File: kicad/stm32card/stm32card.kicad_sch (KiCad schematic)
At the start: 53 parts, among them J1 USB_C_Receptacle_PowerOnly_6P, Q1 AO3400A, U1 MT9216, U2 LM66100DCK, U3 LM66100DCK, U4 STM32F103C8T6, U5 N096-1608TBBIG11-H13

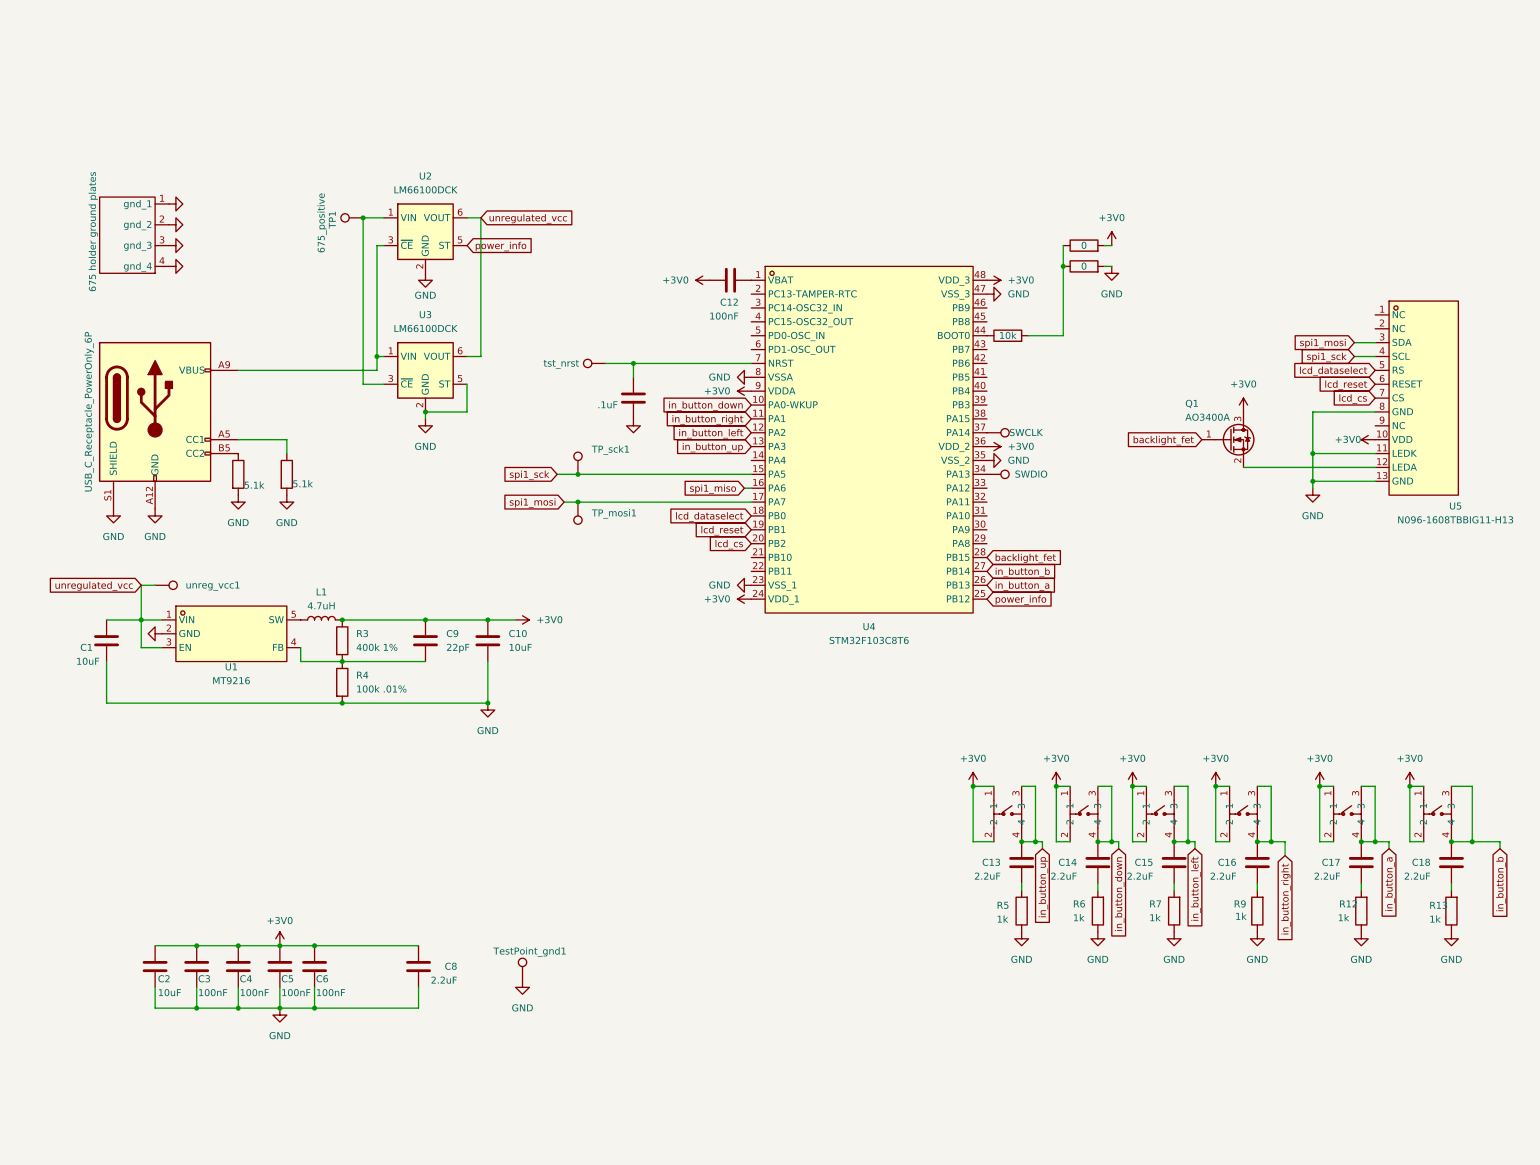
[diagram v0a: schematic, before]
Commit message: need to organize, redid PCB
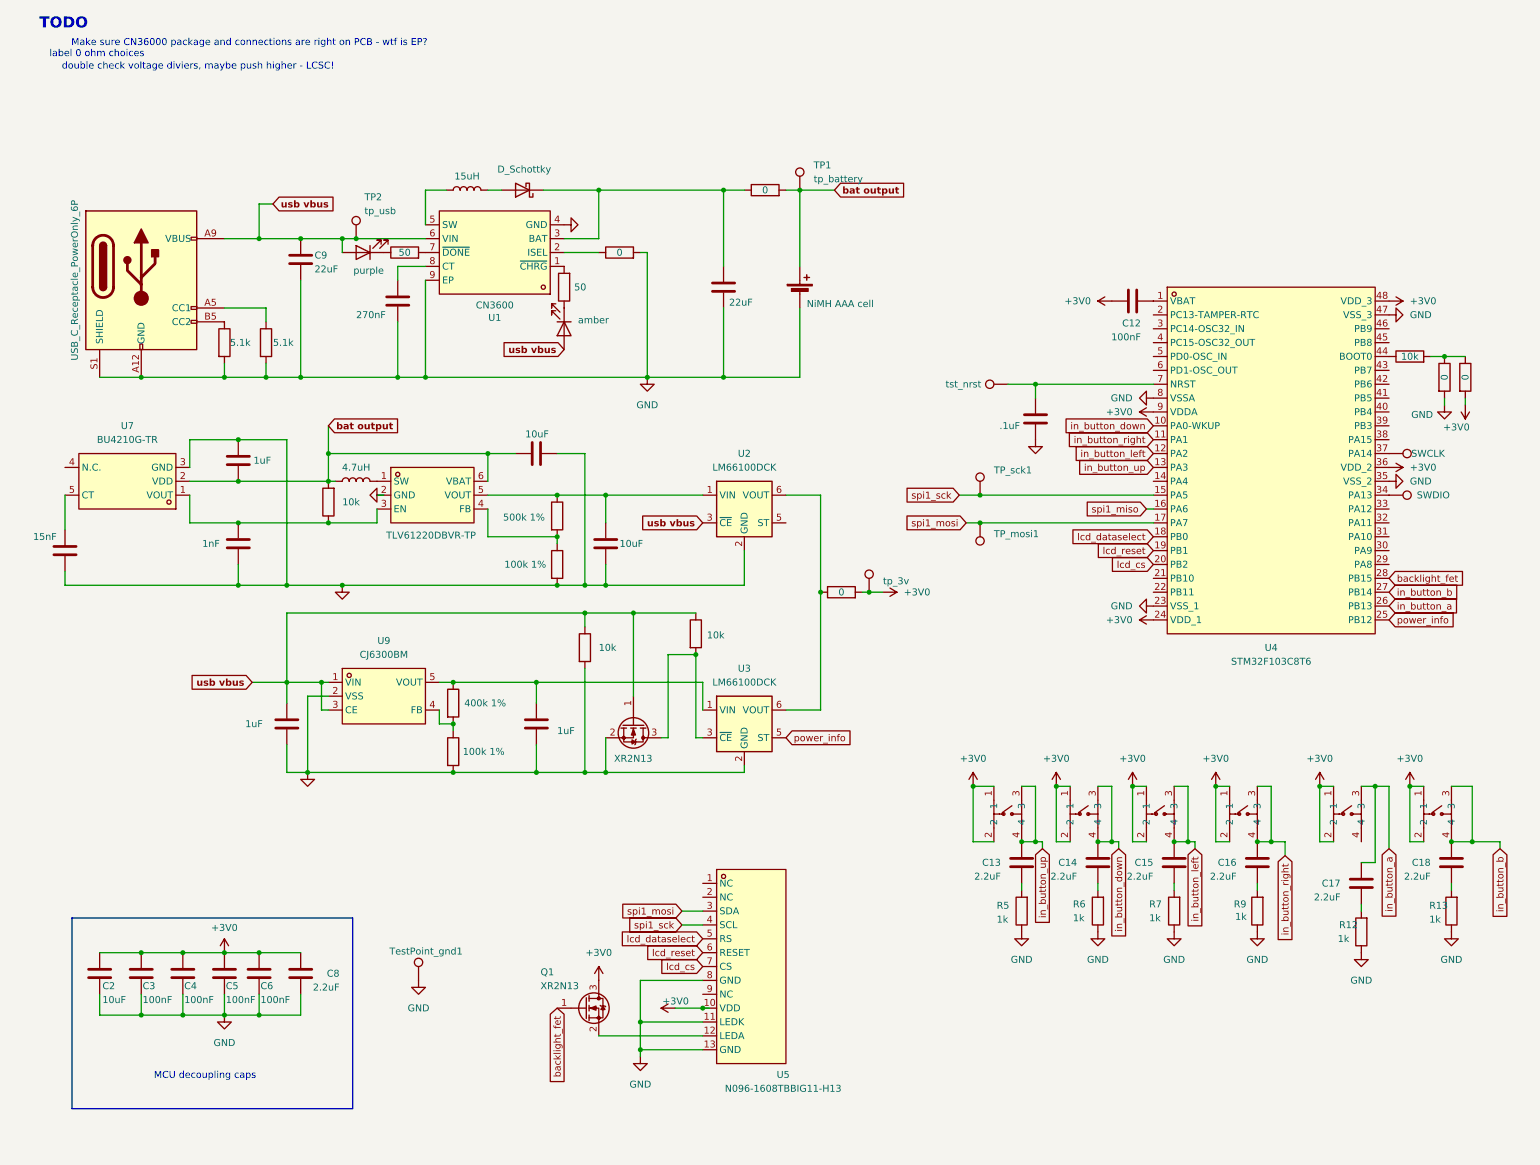
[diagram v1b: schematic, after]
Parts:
- removed R3: 400k 1%, Resistor_SMD:R_0805_2012Metric, symbol Device:R
- removed U1: MT9216, easyeda2kicad:SOT-23-5_L3.0-W1.7-P0.95-LS2.8-BL, symbol easyeda2kicad:MT9216
- removed U6: ~, Library:battery_holder, symbol battery_holder:quad_675
- removed unreg_vcc1: unreg_vcc, TestPoint:TestPoint_Pad_D2.0mm, symbol Connector:TestPoint
- added BT1: NiMH AAA cell, Battery:BatteryHolder_Keystone_2466_1xAAA, symbol Device:Battery_Cell
- added C19: 1nF, Capacitor_SMD:C_0603_1608Metric, symbol Device:C
- added C20, C21, C24: 1uF, Capacitor_SMD:C_0603_1608Metric, symbol Device:C
- added C22, C25: 10uF, Capacitor_SMD:C_0603_1608Metric, symbol Device:C
- added C7: 270nF, Capacitor_SMD:C_0805_2012Metric, symbol Device:C
- added D1: D_Schottky, Diode_SMD:D_SMA, symbol Device:D_Schottky
- added D2: purple, LED_SMD:LED_0805_2012Metric, symbol Device:LED
- added D3: amber, LED_SMD:LED_0603_1608Metric, symbol Device:LED
- added L2: 4.7uH, indigos_imports:IND-SMD_L5.8-W5.2, symbol Device:L
- added Q2: XR2N13, Package_TO_SOT_SMD:SOT-23, symbol Transistor_FET:AO3400A
- added R14, R15: 50, Resistor_SMD:R_0603_1608Metric, symbol Device:R
- added R16: 500k 1%, Resistor_SMD:R_0603_1608Metric, symbol Device:R
- added R17, R19: 100k 1%, Resistor_SMD:R_0603_1608Metric, symbol Device:R
- added R18: 400k 1%, Resistor_SMD:R_0603_1608Metric, symbol Device:R
- added R20, R22, R23: 10k, Resistor_SMD:R_0603_1608Metric, symbol Device:R
- added R21, R24: 0, Resistor_SMD:R_0603_1608Metric, symbol Device:R
- added TP2: tp_usb, TestPoint:TestPoint_Pad_D2.0mm, symbol Connector:TestPoint
- added TP3: tp_3v, TestPoint:TestPoint_Pad_D2.0mm, symbol Connector:TestPoint
- added U1: CN3600, indigos_imports:ESOP-8_L4.9-W3.9-P1.27-LS6.0-BL-EP, symbol indigos_imports:CN3600
- added U6: TLV61220DBVR-TP, indigos_imports:SOT-23-6_L2.9-W1.6-P0.95-LS2.8-BL, symbol indigos_imports:TLV61220DBVR-TP
- added U7: BU4210G-TR, indigos_imports:SSOP-5_L2.9-W1.6-P0.95-LS2.8-TL, symbol indigos_imports:BU4210G-TR
- added U9: CJ6300BM, indigos_imports:SOT-23-5_L2.9-W1.6-P0.95-LS2.8-BR, symbol indigos_imports:CJ6300BM
- C1: value 10uF -> 22uF
- C10: value 10uF -> 15nF
- C9: value 22pF -> 22uF
- L1: value 4.7uH -> 15uH; footprint indigos_kicad_lib:IND-SMD_L5.8-W5.2 -> indigos_imports:IND-SMD_L7.2-W6.6_GPSR07X0
- Q1: value AO3400A -> XR2N13
- R4: value 100k .01% -> 0; footprint Resistor_SMD:R_0805_2012Metric -> Resistor_SMD:R_0603_1608Metric
- TP1: value 675_positive -> tp_battery; footprint TestPoint:TestPoint_Pad_4.0x4.0mm -> TestPoint:TestPoint_Pad_D2.0mm
- TestPoint_gnd1: value TestPoint_gnd -> tp_gnd
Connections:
- net +3V0: now also R24.2, TP3.1; no longer C10.1, C9.1, L1.2
- net GND: now also C9.2, BT1.2 (-), C19.2, C20.1, C21.2, C22.2, C24.2, C25.2, C7.2, Q2.2 (S), R17.2, R19.2, R22.2, U1.4 (GND), U1.9 (EP), U6.2 (GND), U7.3 (GND), U9.2 (VSS); no longer U3.5 (ST)
- net in_button_a: no longer b_a1.4
- net power_info: now also U3.5 (ST); no longer U2.5 (ST)
- net at L1.1: now also U1.5 (SW)
- net usb vbus: now reaches J1.A9 (VBUS), J1.B9 (VBUS), U2.3 (~{CE})
- net usb vbus: now also C9.1, C21.1, D2.2 (A), D3.2 (A), Q2.1 (G), R22.1, R23.1, TP2.1, U1.6 (VIN), U9.1 (VIN), U9.3 (CE); no longer U3.1 (VIN)
- net at R4.1: now also U1.2 (ISEL); no longer C9.2
- net unregulated_vcc: no longer names the net of U2.6 (VOUT), U3.6 (VOUT)
- net unregulated_vcc: now also R24.1; no longer C1.1
- new net: C19.1, R20.1, U6.3 (EN), U7.1 (VOUT)
- new net: D3.1 (K), R15.1
- new net: R15.2, U1.1 (~{CHRG})
- new net: C1.1, D1.1 (K), R21.1, U1.3 (BAT)
- new net: D1.2 (A), L1.2
- new net: D2.1 (K), R14.1
- new net: R18.2, R19.1, U9.4 (FB)
- new net: C24.1, R18.1, U3.1 (VIN), U9.5 (VOUT)
- new net: Q2.3 (D), R23.2, U3.3 (~{CE})
- new net: C22.1, R16.1, U2.1 (VIN), U6.5 (VOUT)
- new net: R16.2, R17.1, U6.4 (FB)
- new net: C7.1, U1.8 (CT)
- new net: C10.1, U7.5 (CT)
- new net: L2.2, U6.1 (SW)
- new net: R14.2, U1.7 (~{DONE})
- new net bat output: BT1.1 (+), C20.2, C25.1, L2.1, R20.2, R21.2, TP1.1, U6.6 (VBAT), U7.2 (VDD)
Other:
- note added: "MCU decoupling caps"
- note added: "Make sure CN36000 package and connections are right on PCB - wtf is EP?"
- note added: "TODO"
- note added: "double check voltage diviers, maybe push higher - LCSC!"
- note added: "label 0 ohm choices"
- moved on the sheet: C12, C17, C2, C3, C4, C5, C6, C8, Q1, R12, TP_mosi1, TP_sck1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

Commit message: quick update for garmin
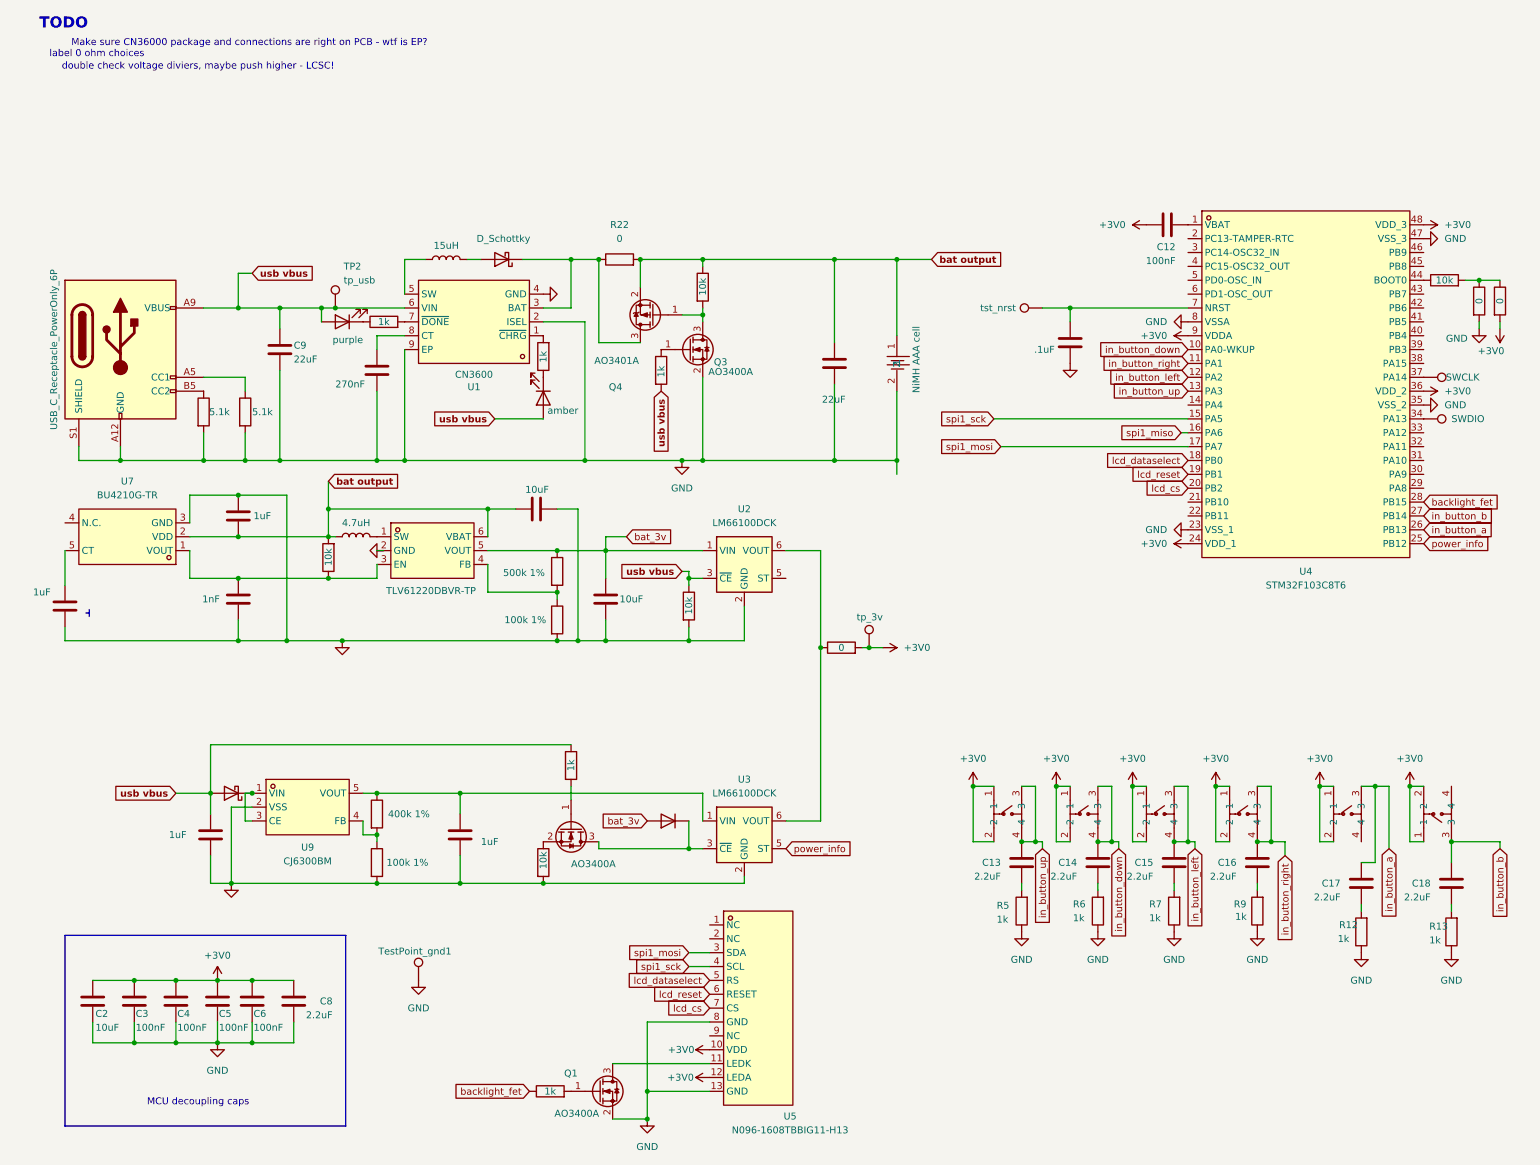
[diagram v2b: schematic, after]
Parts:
- removed TP1: tp_battery, TestPoint:TestPoint_Pad_D2.0mm, symbol Connector:TestPoint
- removed TP_mosi1, TP_sck1: TestPoint, TestPoint:TestPoint_Pad_D2.0mm, symbol Connector:TestPoint
- added D4: D_Schottky, Diode_SMD:D_SMA, symbol Device:D_Schottky
- added D5: 1N4148, Diode_SMD:D_SOD-323, symbol Device:D
- added Q3: AO3400A, Package_TO_SOT_SMD:SOT-23, symbol Transistor_FET:AO3400A
- added Q4: AO3401A, Package_TO_SOT_SMD:SOT-23, symbol Transistor_FET:AO3401A
- added R25: 10k, Resistor_SMD:R_0603_1608Metric, symbol Device:R
- added R26, R3: 1k, Resistor_SMD:R_0603_1608Metric, symbol Device:R
- BT1: footprint Battery:BatteryHolder_Keystone_2466_1xAAA -> indigos_imports:BAT-SMD_BH-AAA-B5BA021; symbol Device:Battery_Cell -> indigos_imports:BH-AAA-B5BA021; LCSC Part (none) -> C7525446
- C10: value 15nF -> 1uF
- Q1, Q2: value XR2N13 -> AO3400A
- R14, R15: value 50 -> 1k
- R21, R4: value 0 -> 10k
- R22: value 10k -> 0
- R23: value 10k -> 1k
- b_a1, b_b1, b_down1, b_left1, b_right1, b_up1: footprint easyeda2kicad:SW-SMD_4P-L6.0-W6.0-P4.50-LS8.6 -> indigos_imports:SW-SMD_4P-L6.0-W6.0-P4.50-LS8.6
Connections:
- net +3V0: now also U5.12 (LEDA); no longer Q1.3 (D)
- net GND: now also Q1.2 (S), R21.2, U1.2 (ISEL), Q3.2 (S); no longer Q2.2 (S), R22.2, U5.11 (LEDK)
- net backlight_fet: now also R26.1; no longer Q1.1 (G)
- net bat output: now also C1.1, R22.2, Q4.2 (S), R25.1; no longer R21.2
- net in_button_b: no longer b_b1.4
- net usb vbus: now also R4.1, D4.2 (A), R3.2; no longer Q2.1 (G), R22.1, U9.1 (VIN), U9.3 (CE)
- net at D1.1 (K), U1.3 (BAT): now also R22.1, Q4.3 (D); no longer C1.1, R21.1
- net at Q2.3 (D), U3.3 (~{CE}): now also D5.1 (K); no longer R23.2
- net bat_3v: now reaches C22.1, R16.1, U2.1 (VIN), U6.5 (VOUT)
- net bat_3v: now also D5.2 (A)
- new net: Q3.1 (G), R3.1
- new net: Q3.3 (D), Q4.1 (G), R25.2
- new net: D4.1 (K), U9.1 (VIN), U9.3 (CE)
- new net: Q1.1 (G), R26.2
- new net: Q1.3 (D), U5.11 (LEDK)
- new net: Q2.1 (G), R23.2
- new net: Q2.2 (S), R21.1
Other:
- moved on the sheet: C12, C18, C2, C3, C4, C5, C6, C8, C9, R13, TP2, U1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
